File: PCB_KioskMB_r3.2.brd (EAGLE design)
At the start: 157 x 103 mm, 340 parts, among them CN2 0039301040, IC1 ISL60002DIH325Z-TK, IC18 FT232RL, IC19 MCP6022-I/ST, IC2 SN65HVD12D, IC20 LTC1771EMS8, IC21 LTC1771EMS8, IC3 PIC24FJ256GA110-I/PT, IC4 PIC10F200T-I/OT, IC5 LM75ADP, IC6 24LC32A-I/MS, IC7 PCF2123TS/1-T, IC8 M25P16-VMN6P, IC9 LM3405AXMK/NOPB, J1 DF11-10DP-2DSA(01), J10 CCM03-3504LFT-NR, J13 3-641215-3, J14 3-641215-2, J15 3-641215-4, J16 3-641215-4, J43 3-641215-4, J44 3-641215-4, J45 3-641215-4, J46 3-641215-5, J47 DF11-10DP-2DSA(01), J48 3-641215-2, J49 3-641215-2, J5 3-641215-2, J6 3-641215-2, J7 SS-6566-NF, J8 TSW-108-07-G-D, J9 SS-6566-NF, Q14 TSM9938HEUK+T, Q15 SI4564DY, Q16 CSD87331Q3D, Q17 TSM9938HEUK+T, Q18 SI4564DY, Q19 CSD87331Q3D, Q2 FDC6330L, Q20 IPD30N06S2L-23, Q21 IPD30N06S2L-23, Q22 FDN352AP, Q23 FDN352AP, Q24 BSS138, Q3 SR3.3.TCT, Q4 7B-28.63636MAAJ-T, Q5 FDC6324L, Q6 CM519 32.768KDZF-UT, Q7 SSM6P49NU,LFPZ, Q8 IPD30N06S2L-23, Q9 IPD30N06S2L-23, U1 LTC1955, U2 HRXL-MAXSONAR-WRC-MB7387, U3 ADS1015, U6 TPS43061, U7 TPS43061, U8 TPA3111D1PWP, U9 OPA322SAIDBVT, X1 FH12-10S-0.5S1.00MM, X2 MINI-USB_4P-85-32004-10X

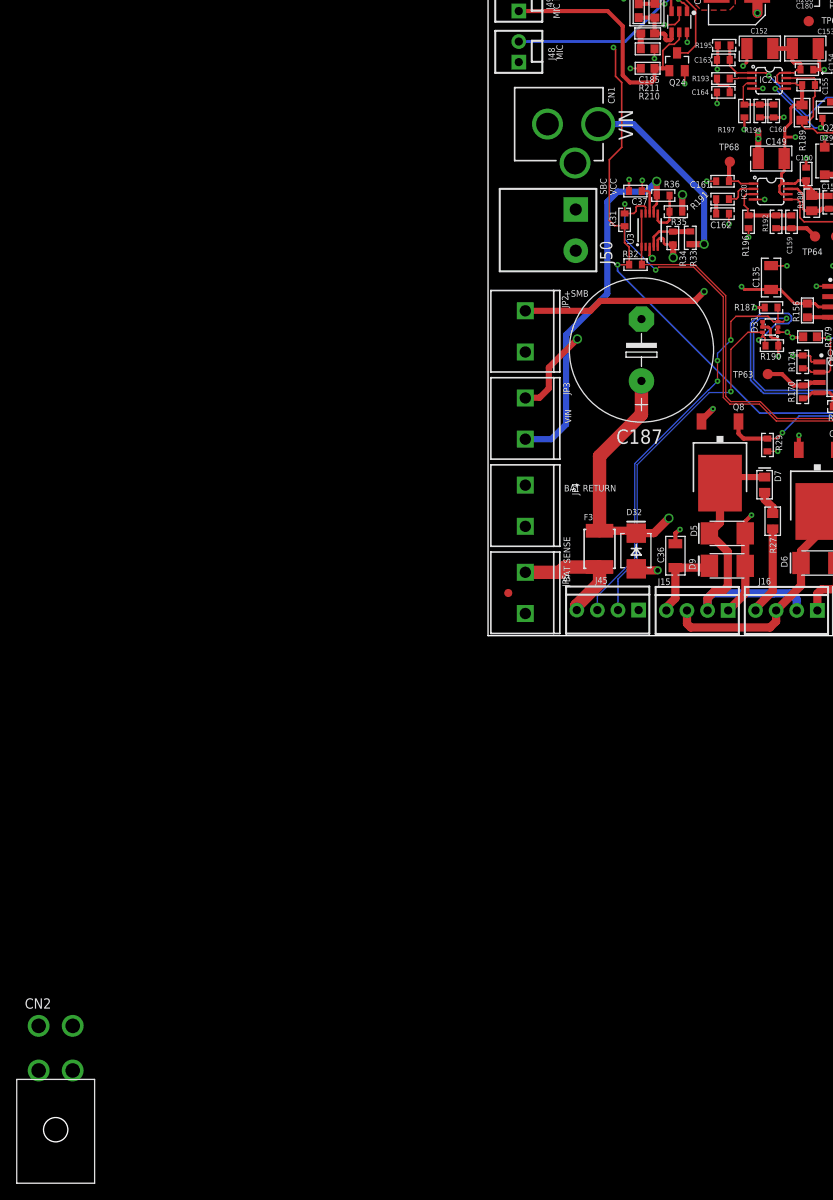
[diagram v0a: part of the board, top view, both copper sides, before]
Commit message: push latest
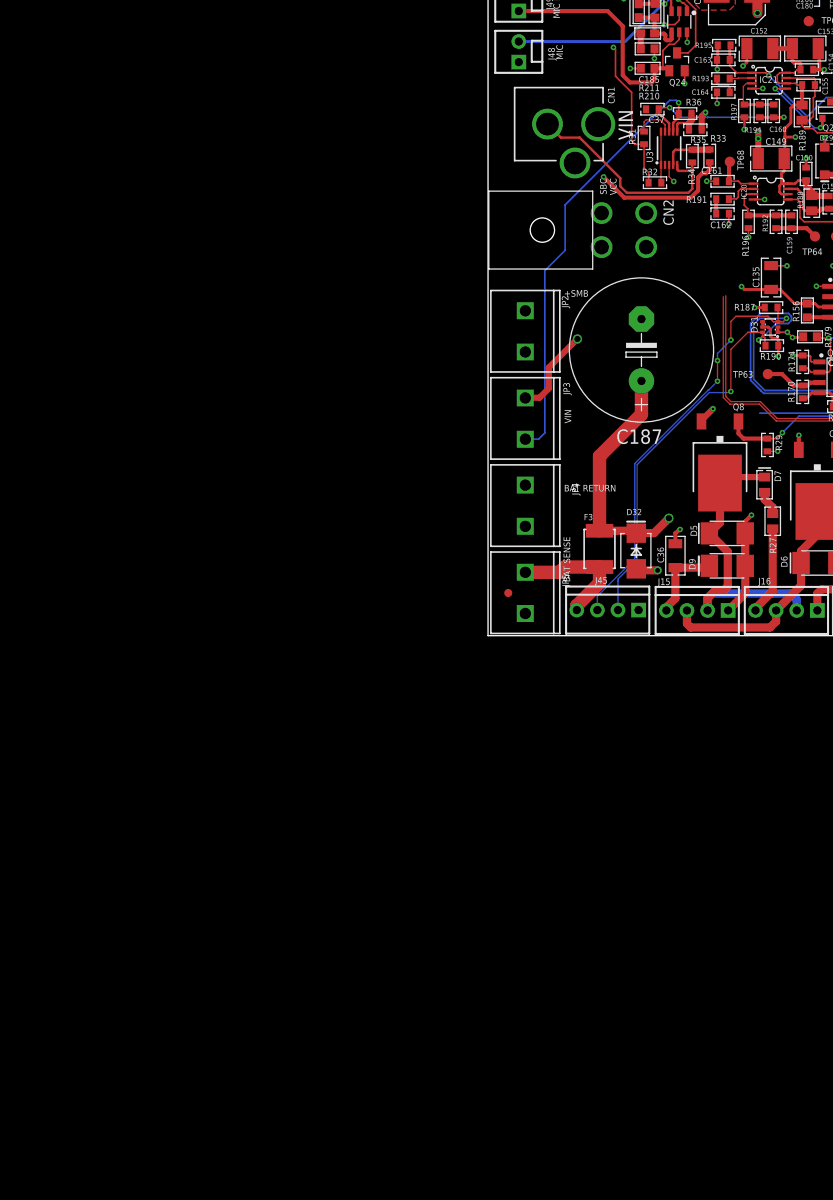
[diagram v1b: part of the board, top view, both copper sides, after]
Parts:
- removed J50: (no value), CON-PhoenixContac-AON:TERM-2
- moved CN2 123.5 mm to (14.0, 50.0), turned to 270 degrees
- moved R36 10.5 mm to (24.3, 64.4)
- moved R31 10.4 mm to (19.2, 61.4)
- moved R32 10.4 mm to (20.6, 55.8)
- moved R33 10.4 mm to (27.3, 59.1)
- moved R34 10.4 mm to (25.2, 59.1)
- moved R35 10.4 mm to (25.6, 62.4)
- moved U3 10.4 mm to (22.3, 60.1)
- moved C37 10.3 mm to (20.3, 64.9)
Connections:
- net DGND: now also CN2.1, CN2.2; no longer J50.1
- net P12V: now also CN2.3, CN2.4; no longer J50.2
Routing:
- net +3.3V/1: track 275.1 -> 237.7 mm, vias 7 -> 6
- net SDA1: track 223.6 -> 203.6 mm, vias 10 -> 8
- net SCL1: track 205.2 -> 193.3 mm
- net BAT_SENSE: track 50.6 -> 62.2 mm
- net BAT_GND: track 61.2 -> 69.8 mm
- net P12V: track 170.0 -> 161.5 mm
- net +5V: track 75.2 -> 67.2 mm
- net 18V_SENSE: track 53.3 -> 50.0 mm, vias 2 -> 1
- net 18V_GND: track 63.0 -> 60.5 mm, vias 1 -> 0
- net N$21: track 5.57 -> 4.55 mm
- net DGND: track 402.4 -> 401.6 mm, vias 137 -> 136
